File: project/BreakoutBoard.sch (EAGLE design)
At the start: 2 parts, among them J1 XF2L-2435-1, X1 LCD

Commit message: Layout complete
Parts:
- added B1: RESET, alps:SKSCLDE010
- added B2: BOOT, alps:SKSCLDE010
- added C1: 22pF/50V, SparkFun-Capacitors:22PF-0402T-16V-10%
- added C105: 2.2uF/16V, rcl:C-EUC0603
- added C106: 4.7uF/16V, rcl:C-EUC0603
- added C107: 22pF/50V, rcl:C-EUC0402
- added C17: 10uF/16V, rcl:C-EUC0603
- added C18: 0.1uF/10V, rcl:C-EUC0402
- added C19: 1uF/16V, rcl:C-EUC0402
- added C2, C5: 10uF/16V, SparkFun-Capacitors:10UF-0603-6.3V-20%
- added C3, C4: 0.1uF/10V, SparkFun-Capacitors:0.1UF-0402-10V-10%-X7R
- added C86: (no value), rcl:C-EUC0402
- added CN2: (no value), adafruit:JST_2PIN-SMT
- added D1, D15: (no value), diode:DIODE-SOD123
- added D10, D8, D9: LESD5D5.0CT1G, discrete:LESD5D5.0CT1G
- added D11, D12, D2: LESD8D3.3CAT5G, discrete:LESD8D3.3CAT5G
- added D19: (no value), adafruit:DIODESOD-523
- added D3: (no value), led:LEDCHIPLED_1206
- added J2: I2C2, SparkFun-Connectors:QWIIC_CONNECTOR
- added J3: LCD, ER-CON0.4-24P:ER-CON0.4-24
- added L1: 2.2μH, SparkFun-Coils:2.2μH-4X4-2.2μH-3A-45MOHM
- added L6: 10uH_0.8A, discrete:SRN3010TA
- added R1, R13: 10K, rcl:R-US_R0402
- added R111, R112: 0, rcl:R-US_R0201
- added R12, R123: 0, rcl:R-US_R0603
- added R126: 6.6, rcl:R-US_R0402
- added R127: 10, rcl:R-US_R0402
- added R2: 680K, rcl:R-US_R0402
- added R3: 150K, rcl:R-US_R0402
- added R74: 51, rcl:R-US_R0201
- added TP1, TP2: TEST-POINT3, SparkFun-Connectors:TEST-POINT3
- added U1: SY8088, discrete:SY8088
- added U15: BD60A60NUX, discrete:BD60A60NUX
- added U4: ESP32-S3-WROOM-1, espressif:ESP32-S3-WROOM-1
- J1: value XF2L-2435-1 -> I2C1; device con-omron:XF2L-2435-1 -> SparkFun-Connectors:QWIIC_CONNECTOR
- X1: value LCD -> (none); device ER-CON0.4-24P:ER-CON0.4-24 -> Adafruit ItsyBitsy nRF52840 Express:MICROBUILDER_USBMICRO_20329
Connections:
- removed net N$10: J1-10.MS, X1-10.1
- removed net N$11: J1-11.MS, X1-11.1
- removed net N$12: J1-12.MS, X1-12.1
- removed net N$13: J1-13.MS, X1-13.1
- removed net N$14: J1-14.MS, X1-14.1
- removed net N$15: J1-15.MS, X1-15.1
- removed net N$16: J1-16.MS, X1-16.1
- removed net N$17: J1-17.MS, X1-17.1
- removed net N$18: J1-18.MS, X1-18.1
- removed net N$19: J1-19.MS, X1-19.1
- removed net N$20: J1-20.MS, X1-20.1
- removed net N$21: J1-21.MS, X1-21.1
- removed net N$22: J1-22.MS, X1-22.1
- removed net N$23: J1-23.MS, X1-23.1
- removed net N$24: J1-24.MS, X1-24.1
- removed net N$3: J1-3.MS, X1-3.1
- removed net N$5: J1-5.MS, X1-5.1
- new net ESP_3V3: C17.1, C18.1, D2.C, R12.2, R13.1, U4.3V3
- new net GND: B1.1, B2.1, C105.2, C106.2, C107.2, C17.2, C18.2, C19.2, C2.2, C3.2, C4.2, C5.2, C86.2, CN2.1, D10.A, D11.A, D12.A, D2.A, D8.A, D9.A, J1.1, J2.1, J3-15.1, J3-16.1, J3-3.1, J3-4.1, R123.1, R126.1, R3.1, R74.1, TP2.1, U1.GND, U15.GND, U4.EPAD, U4.GND, U4.GND1
- new net GPIO0: B2.4, D12.C, U4.IO0
- new net GPIO18: J1.4, U4.IO18
- new net GPIO19: R111.2, U4.IO19
- new net GPIO20: R112.2, U4.IO20
- new net GPIO3: J3-21.1, U4.IO3
- new net GPIO4: J3-5.1, U4.IO4
- new net GPIO40: J2.4, J3-20.1, U4.IO40
- new net GPIO41: J2.3, J3-19.1, U4.IO41
- new net GPIO45: R127.1, U4.IO45
- new net GPIO48: J3-10.1, J3-18.1, U15.EN, U4.IO48
- new net GPIO5: J3-9.1, U4.IO5
- new net GPIO6: J3-8.1, U4.IO6
- new net GPIO7: J3-6.1, U4.IO7
- new net GPIO8: J1.3, U4.IO8
- new net LED_A: C105.1, D19.C, J3-23.1, J3-24.1, U15.VOUT
- new net LED_DIM: C107.1, R127.2, U15.PWM
- new net LED_K: J3-1.1, J3-2.1, U15.FB
- new net MCU_RST: B1.4, C19.1, D11.C, R13.2, U4.EN
- new net MCU_VDD: C1.1, C4.1, C5.1, C86.1, D3.A, J1.2, J2.2, J3-11.1, J3-12.1, J3-13.1, J3-14.1, J3-17.1, L1.2, R12.1, R2.2, TP1.1
- new net USB_5V: C106.1, C2.1, C3.1, D1.C, D15.C, L6.1, R1.1, U1.IN, U15.VIN
- new net USB_DN: D9.C, R111.1, X1.D-
- new net USB_DP: D10.C, R112.1, X1.D+
- new net USB_G: R123.2, X1.GND
- new net USB_VBUS: D1.A, D8.C, X1.VBUS
- net N$1: now also D19.A, L6.2, U15.SW; no longer J1-1.MSV, X1-1.1
- net N$2: now also D3.C, R74.2; no longer J1-2.MS, X1-2.1
- net N$4: now also CN2.2, D15.A; no longer J1-4.MS, X1-4.1
- net N$6: now also R1.2, U1.EN; no longer J1-6.MS, X1-6.1
- net N$7: now also L1.1, U1.LX; no longer J1-7.MS, X1-7.1
- net N$8: now also C1.2, R2.1, R3.2, U1.FB; no longer J1-8.MS, X1-8.1
- net N$9: now also R126.2, U15.ISET; no longer J1-9.MS, X1-9.1

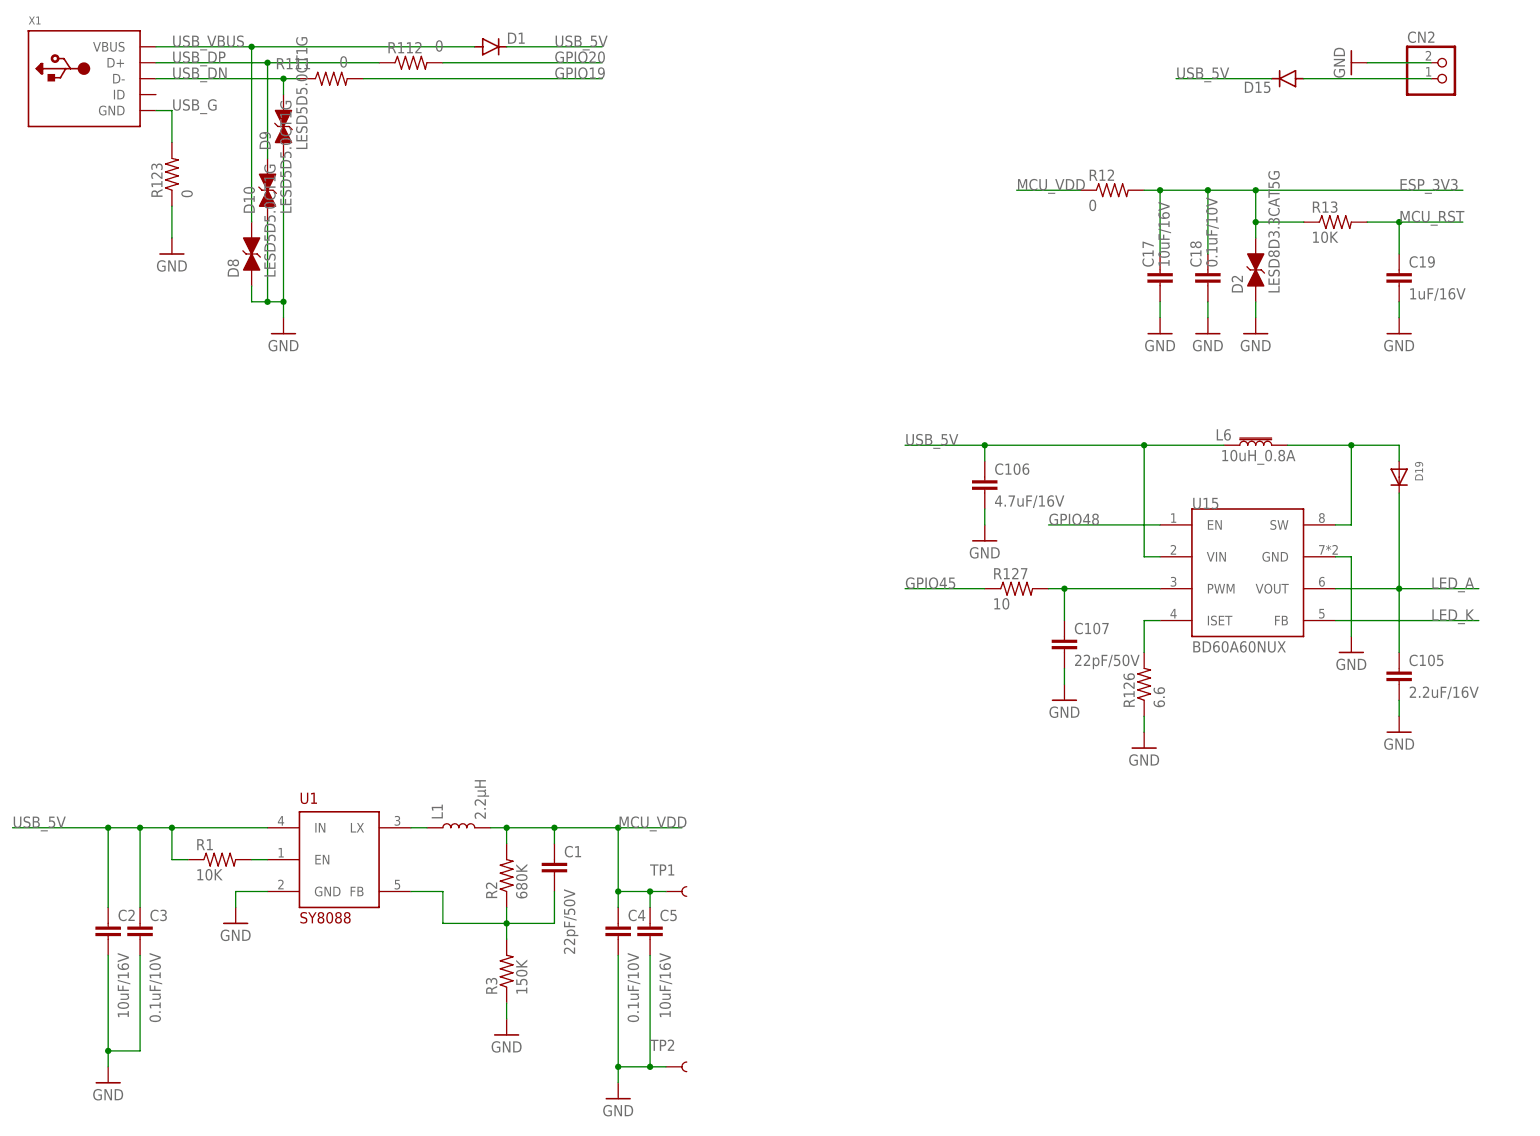
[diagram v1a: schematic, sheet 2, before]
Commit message: Layout optimization
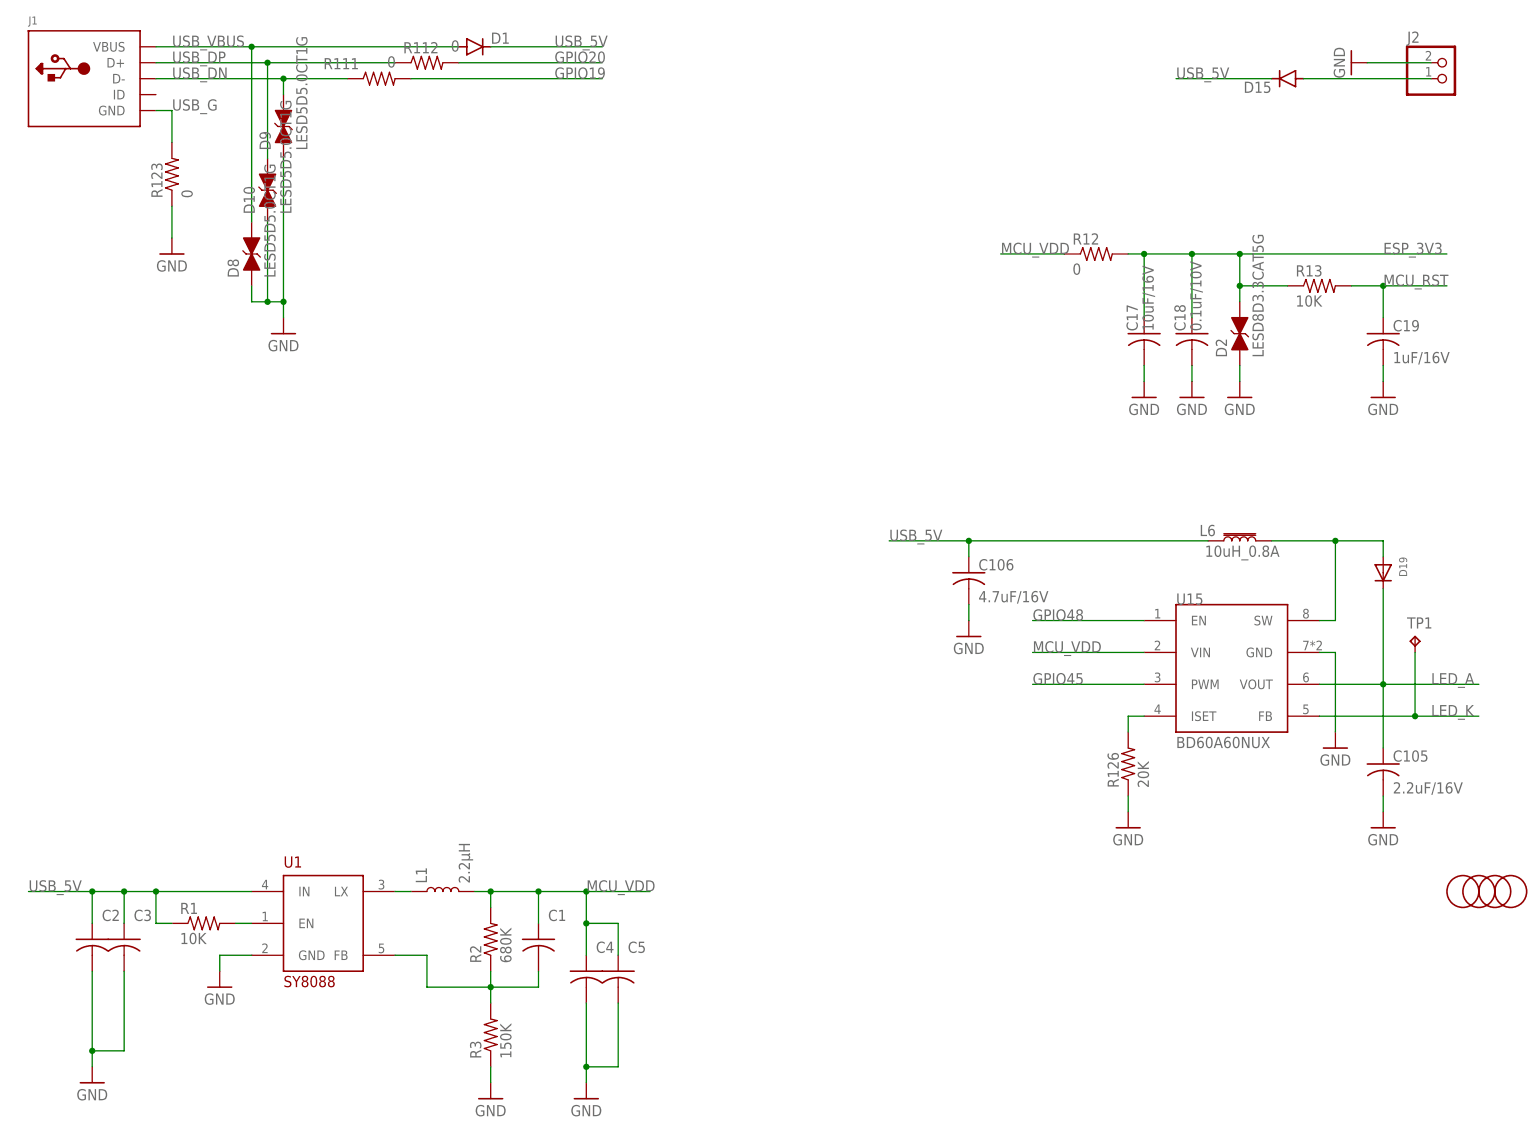
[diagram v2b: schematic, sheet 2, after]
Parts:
- removed C107: 22pF/50V, rcl:C-EUC0402
- removed CN2: (no value), adafruit:JST_2PIN-SMT
- removed R127: 10, rcl:R-US_R0402
- removed TP2: TEST-POINT3, SparkFun-Connectors:TEST-POINT3
- removed X1: (no value), Adafruit ItsyBitsy nRF52840 Express:MICROBUILDER_USBMICRO_20329
- added C97: 0.1uF/6.3V, rcl:C-USC0402
- added C98: 4.7uF/6.3V, rcl:C-USC0402
- added J4: I2C1, SparkFun-Connectors:QWIIC_CONNECTOR
- added J5: I2C2, SparkFun-Connectors:QWIIC_CONNECTOR
- added U$1, U$2, U$4, U$5: FIDUCIAL, adafruit:FIDUCIAL
- B1, B2: LCSC (none) -> C115362
- C1: device SparkFun-Capacitors:22PF-0402T-16V-10% -> rcl:C-USC0402; LCSC (none) -> C106203
- C105: device rcl:C-EUC0603 -> rcl:C-USC0603; LCSC (none) -> C106853
- C106: device rcl:C-EUC0603 -> rcl:C-USC0603; LCSC (none) -> C277476
- C17: device rcl:C-EUC0603 -> rcl:C-USC0603; LCSC (none) -> C86275
- C18: device rcl:C-EUC0402 -> rcl:C-USC0402; LCSC (none) -> C161163
- C19: device rcl:C-EUC0402 -> rcl:C-USC0402; LCSC (none) -> C77007
- C2: device SparkFun-Capacitors:10UF-0603-6.3V-20% -> rcl:C-USC0603; LCSC (none) -> C86275
- C3: device SparkFun-Capacitors:0.1UF-0402-10V-10%-X7R -> rcl:C-USC0603; LCSC (none) -> C161163
- C4: device SparkFun-Capacitors:0.1UF-0402-10V-10%-X7R -> rcl:C-USC0402; LCSC (none) -> C161163
- C5: device SparkFun-Capacitors:10UF-0603-6.3V-20% -> rcl:C-USC0402; LCSC (none) -> C86275
- C86: value (none) -> 0.1uF/6.3V; device rcl:C-EUC0402 -> rcl:C-USC0402; LCSC (none) -> C541406
- D1, D15: LCSC (none) -> C511872
- D10, D8, D9: LCSC (none) -> C383211
- D11, D12, D2: LCSC (none) -> C172409
- D19: LCSC (none) -> C253516
- D3: LCSC (none) -> C375534
- J1: value I2C1 -> (none); device SparkFun-Connectors:QWIIC_CONNECTOR -> Adafruit ItsyBitsy nRF52840 Express:MICROBUILDER_USBMICRO_20329; LCSC (none) -> C40946
- J2: value I2C2 -> (none); device SparkFun-Connectors:QWIIC_CONNECTOR -> adafruit:JST_2PIN-SMT; LCSC (none) -> C64658
- L1: LCSC (none) -> C370436
- L6: LCSC (none) -> C518881
- R1, R13: LCSC (none) -> C60490
- R111, R112: LCSC (none) -> C106227
- R12, R123: LCSC (none) -> C100044
- R126: value 6.6 -> 20K; LCSC (none) -> C326980
- R2: LCSC (none) -> C163456
- R3: LCSC (none) -> C93947
- R74: LCSC (none) -> C163499
- TP1: value TEST-POINT3 -> TPTP06R; device SparkFun-Connectors:TEST-POINT3 -> testpad:TPTP06R
- U1: LCSC (none) -> C79313
- U15: LCSC (none) -> C2678724
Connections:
- removed net LED_DIM: C107.1, R127.2, U15.PWM
- net GND: now also B1.2, B2.2, C97.2, C98.2, J4.1, J5.1; no longer C107.2, CN2.1, J1.1, TP2.1
- net GPIO0: now also B2.3
- net GPIO18: now also J4.4; no longer J1.4
- net GPIO40: now also J5.4; no longer J2.4
- net GPIO41: now also J5.3; no longer J2.3
- net GPIO45: now also U15.PWM; no longer R127.1
- net GPIO8: now also J4.3; no longer J1.3
- net LED_K: now also TP1.TP
- net MCU_RST: now also B1.3
- net MCU_VDD: now also C97.1, C98.1, J4.2, J5.2, U15.VIN; no longer J1.2, J2.2, TP1.1
- net N$4: now also J2.2; no longer CN2.2
- net USB_5V: no longer U15.VIN
- net USB_DN: now also J1.D-; no longer X1.D-
- net USB_DP: now also J1.D+; no longer X1.D+
- net USB_G: now also J1.GND; no longer X1.GND
- net USB_VBUS: now also J1.VBUS; no longer X1.VBUS
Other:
- moved on the sheet: B1, B2, C1, C105, C106, C17, C18, C19, C2, C3, C4, C5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
